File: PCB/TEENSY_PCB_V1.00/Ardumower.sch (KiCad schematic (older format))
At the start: 50 parts, among them J1 ODO_Left, J10 Sonar_R, J11 Cutter, J12 Sonar_L, J13 P_Right, J14 Buzzer, J15 Button, J16 Power_Board, J19 P_Left, J2 I2C2_0, J25 5V IN, J29 3.3V IN, J3 I2C0_0, J30 I2C1_0, J31 Ser3, J4 I2C1_1, J5 Bumper, J6 ODO_Right, J7 Motor_Right1, J8 Motor_Left1, J9 Rain, U1 DOIT-ESP32-DEVKIT-V1, U2 GY-521, U3 Teensy4.1

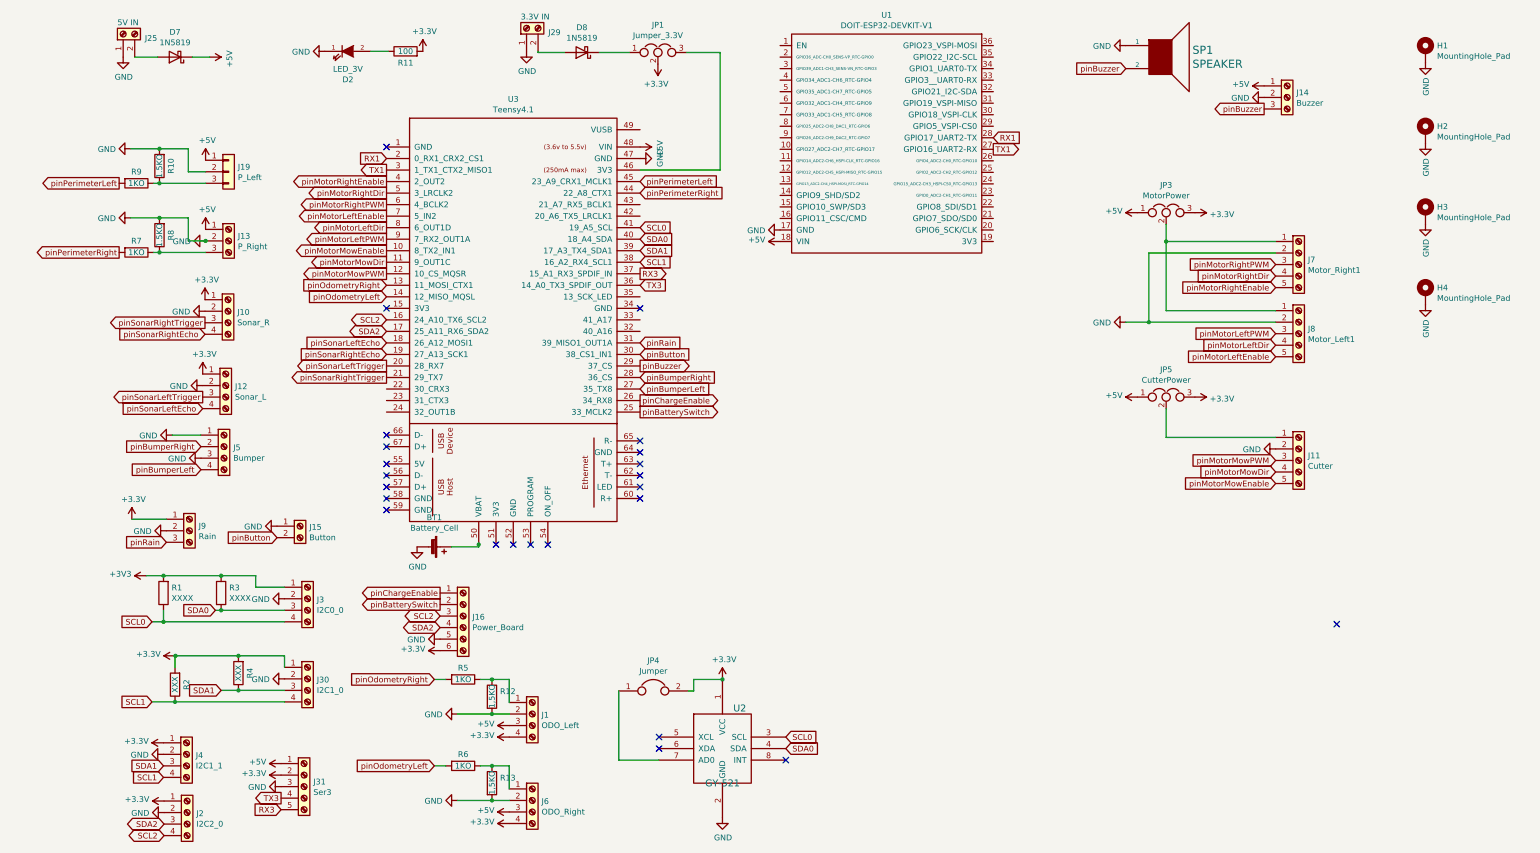
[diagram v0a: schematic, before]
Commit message: teensy pcb
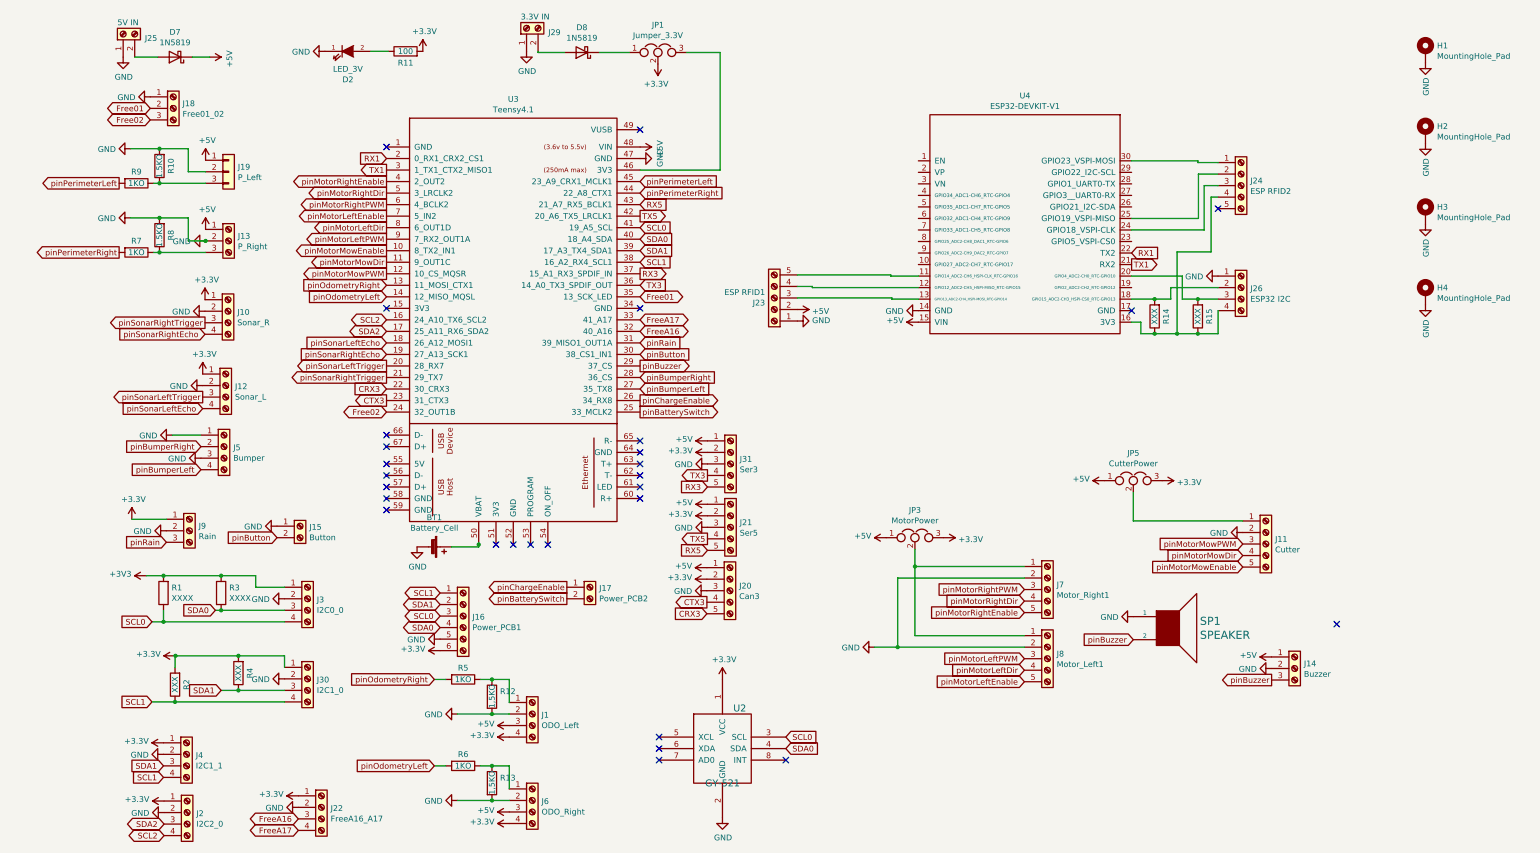
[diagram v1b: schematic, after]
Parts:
- removed JP4: Jumper, Connector_PinSocket_2.54mm:PinSocket_1x02_P2.54mm_Vertical, symbol Device:Jumper
- removed U1: DOIT-ESP32-DEVKIT-V1, teensy_library-master:ESP32-DOIT-DEVKIT, symbol doit-esp32-devkit-v1:DOIT-ESP32-DEVKIT-V1
- added J17: Power_PCB2, Connector_JST:JST_XH_B2B-XH-A_1x02_P2.50mm_Vertical, symbol Connector:Screw_Terminal_01x02
- added J18: Free01_02, Connector_JST:JST_XH_B3B-XH-A_1x03_P2.50mm_Vertical, symbol Connector:Screw_Terminal_01x03
- added J20: Can3, Connector_JST:JST_XH_B5B-XH-A_1x05_P2.50mm_Vertical, symbol Connector:Screw_Terminal_01x05
- added J21: Ser5, Connector_JST:JST_XH_B5B-XH-A_1x05_P2.50mm_Vertical, symbol Connector:Screw_Terminal_01x05
- added J22: FreeA16_A17, Connector_JST:JST_XH_B4B-XH-A_1x04_P2.50mm_Vertical, symbol Connector:Screw_Terminal_01x04
- added J23: ESP RFID1, Connector_JST:JST_XH_B5B-XH-A_1x05_P2.50mm_Vertical, symbol Connector:Screw_Terminal_01x05
- added J24: ESP RFID2, Connector_JST:JST_XH_B5B-XH-A_1x05_P2.50mm_Vertical, symbol Connector:Screw_Terminal_01x05
- added J26: ESP32 I2C, Connector_JST:JST_XH_B4B-XH-A_1x04_P2.50mm_Vertical, symbol Connector:Screw_Terminal_01x04
- added R14, R15: XXX, Resistor_THT:R_Axial_DIN0207_L6.3mm_D2.5mm_P2.54mm_Vertical, symbol Device:R
- added U4: ESP32-DEVKIT-V1, teensy_library-master:ESP32-DEVKIT-V1, symbol teensy:ESP32-DEVKIT-V1
- J16: value Power_Board -> Power_PCB1
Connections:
- net +3V3: now also J20.2 (Pin_2), J21.2 (Pin_2), J22.1 (Pin_1)
- net +5V: now also J20.1 (Pin_1), J21.1 (Pin_1), J23.2 (Pin_2), U4.15 (VIN)
- net GND: now also J18.1 (Pin_1), J20.3 (Pin_3), J21.3 (Pin_3), J22.2 (Pin_2), J23.1 (Pin_1), J26.1 (Pin_1), U4.14 (GND)
- net RX1: now also U4.22 (TX2)
- net SCL0: now also J16.3 (Pin_3)
- net SCL1: now also J16.1 (Pin_1)
- net SCL2: no longer J16.3 (Pin_3)
- net SDA0: now also J16.4 (Pin_4)
- net SDA1: now also J16.2 (Pin_2)
- net SDA2: no longer J16.4 (Pin_4)
- net TX1: now also U4.21 (RX2)
- net pinBatterySwitch: now also J17.2 (Pin_2); no longer J16.2 (Pin_2)
- net pinChargeEnable: now also J17.1 (Pin_1); no longer J16.1 (Pin_1)
- net CRX3: now reaches U3.22 (30_CRX3)
- net CRX3: now also J20.5 (Pin_5)
- net CTX3: now reaches U3.23 (31_CTX3)
- net CTX3: now also J20.4 (Pin_4)
- net Free02: now reaches U3.24 (32_OUT1B)
- net Free02: now also J18.3 (Pin_3)
- net FreeA16: now reaches U3.32 (40_A16)
- net FreeA16: now also J22.3 (Pin_3)
- net FreeA17: now reaches U3.33 (41_A17)
- net FreeA17: now also J22.4 (Pin_4)
- net Free01: now reaches U3.35 (13_SCK_LED)
- net Free01: now also J18.2 (Pin_2)
- net TX5: now reaches U3.42 (20_A6_TX5_LRCLK1)
- net TX5: now also J21.4 (Pin_4)
- net RX5: now reaches U3.43 (21_A7_RX5_BCLK1)
- net RX5: now also J21.5 (Pin_5)
- new net: J23.5 (Pin_5), U4.11 (GPIO14_ADC2-CH6_HSPI-CLK_RTC-GPIO16)
- new net: J23.4 (Pin_4), U4.12 (GPIO12_ADC2-CH5_HSPI-MISO_RTC-GPIO15)
- new net: J23.3 (Pin_3), U4.13 (GPIO13_ADC2-CH4_HSPI-MOSI_RTC-GPIO14)
- new net: J24.4 (Pin_4), J26.4 (Pin_4), R14.1, R15.1, U4.16 (3V3)
- new net: J26.2 (Pin_2), R14.2, U4.18 (GPIO15_ADC2-CH3_HSPI-CS0_RTC-GPIO13)
- new net: J26.3 (Pin_3), R15.2, U4.20 (GPIO4_ADC2-CH0_RTC-GPIO10)
- new net: J24.3 (Pin_3), U4.24 (GPIO18_VSPI-CLK)
- new net: J24.2 (Pin_2), U4.25 (GPIO19_VSPI-MISO)
- new net: J24.1 (Pin_1), U4.30 (GPIO23_VSPI-MOSI)
- no-connect marks 24 -> 28
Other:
- moved on the sheet: J11, J14, J31, J7, J8, JP3, JP5, SP1
